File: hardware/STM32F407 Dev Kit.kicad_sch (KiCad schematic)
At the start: 0 parts

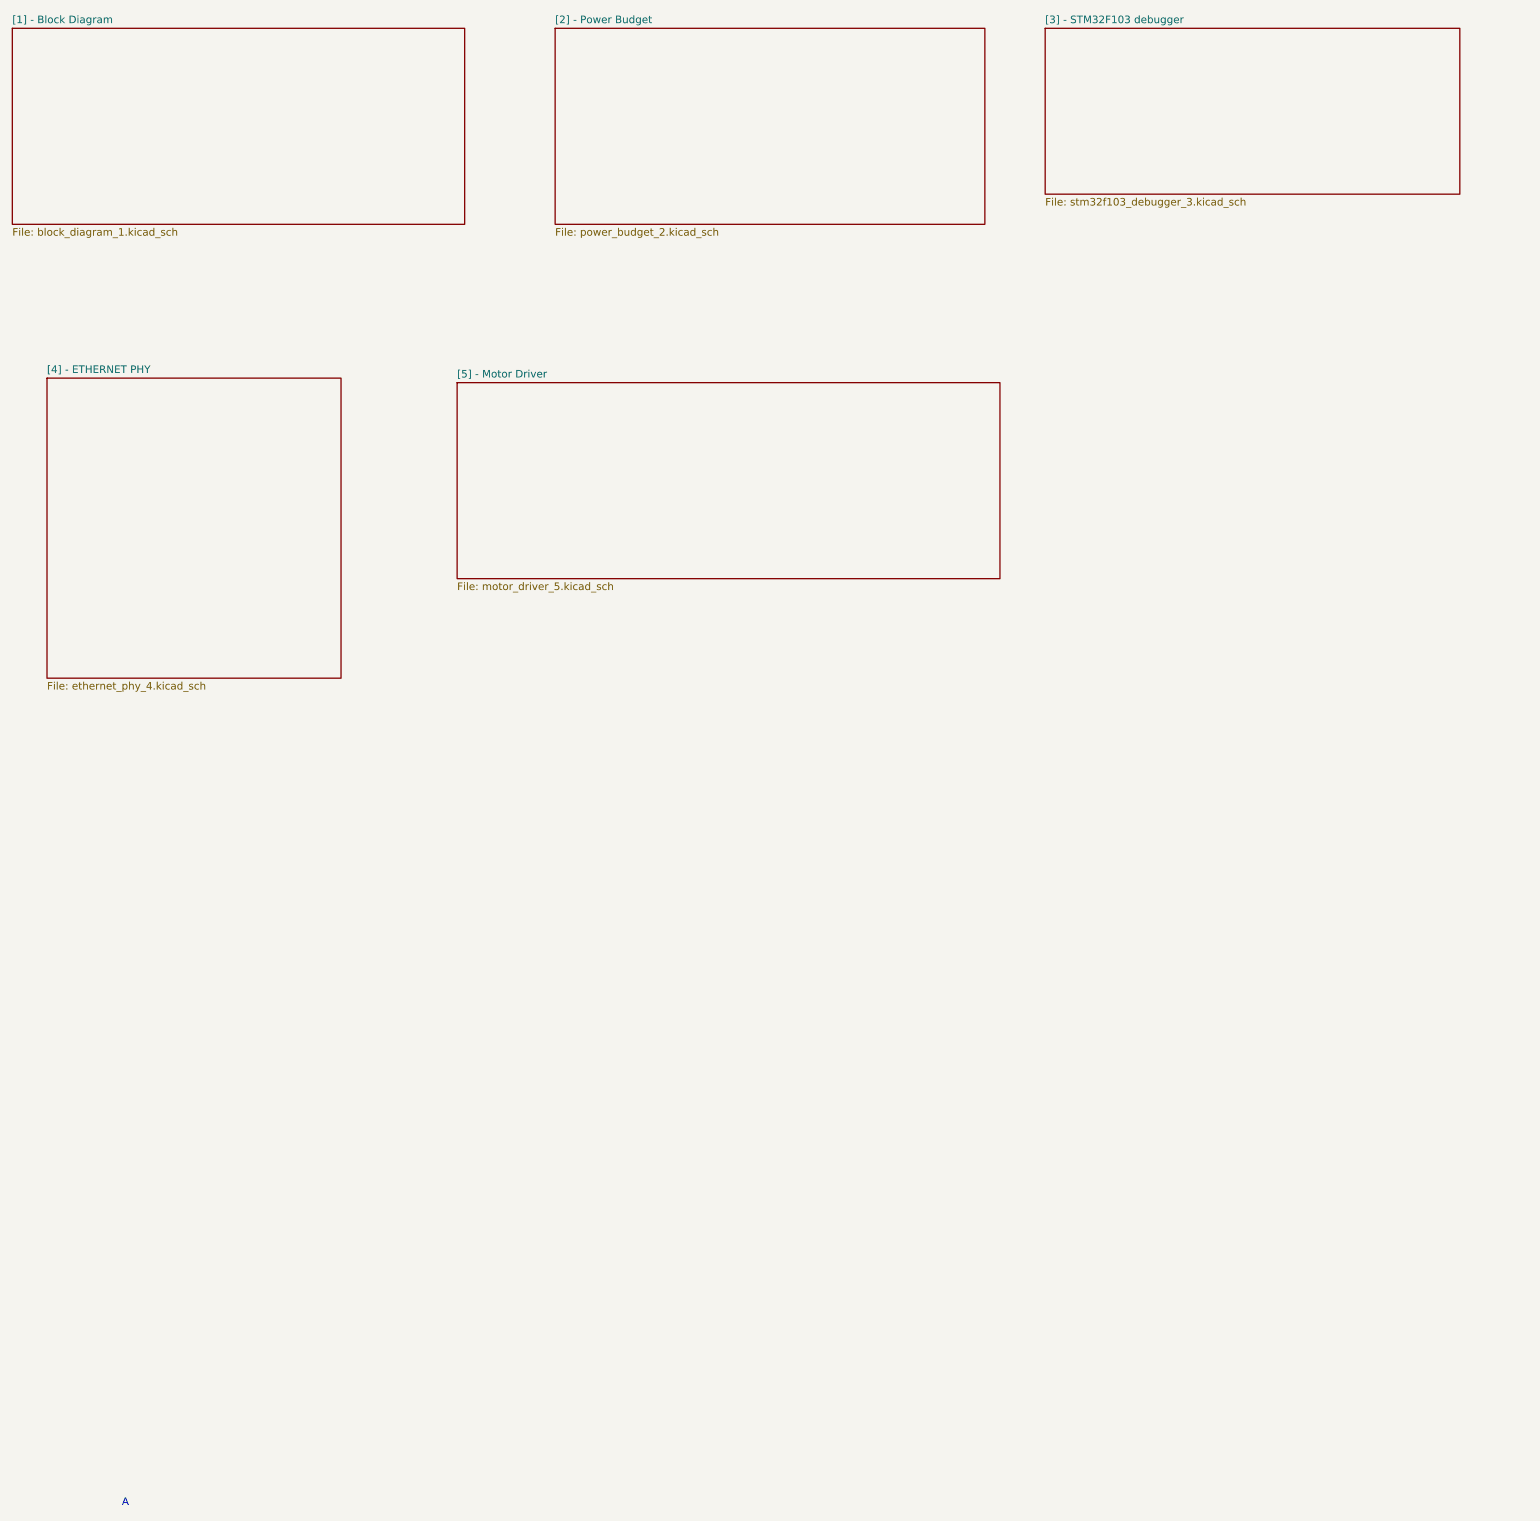
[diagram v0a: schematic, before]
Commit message: Design schematic for MIC & Headphones
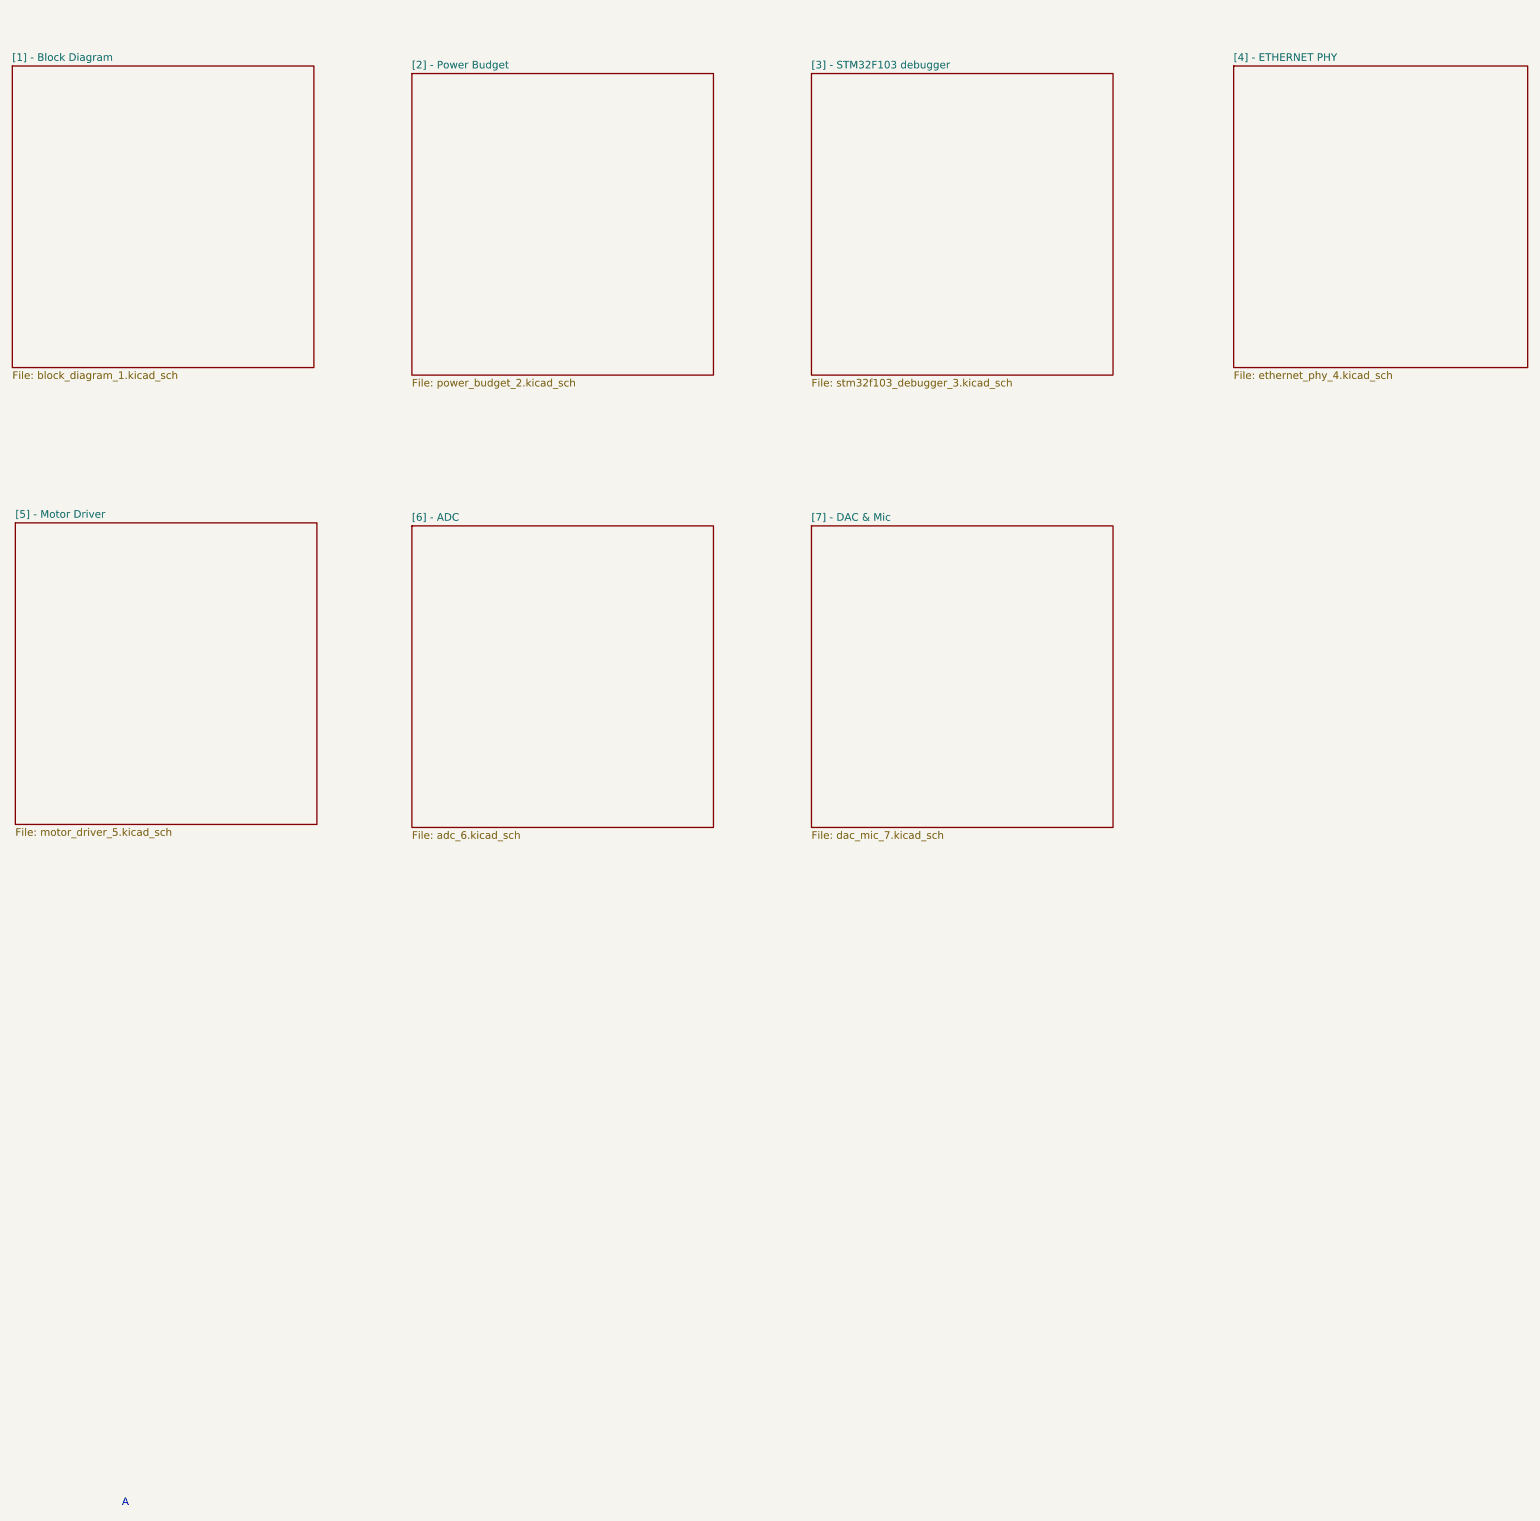
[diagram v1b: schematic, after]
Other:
- added sheet [6] - ADC (adc_6.kicad_sch)
- added sheet [7] - DAC & Mic (dac_mic_7.kicad_sch)
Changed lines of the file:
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@@
 	)
 	(sheet
-		(at 20.32 17.78)
-		(size 76.2 33.02)
+		(at 20.32 24.13)
+		(size 50.8 50.8)
 		(exclude_from_sim no)
 		(in_bom yes)
@@
 		)
 		(property "Sheetname" "[1] - Block Diagram"
-			(at 20.32 17.0684 0)
+			(at 20.32 23.4184 0)
 			(show_name no)
 			(do_not_autoplace no)
@@
 		)
 		(property "Sheetfile" "block_diagram_1.kicad_sch"
-			(at 20.32 51.3846 0)
+			(at 20.32 75.5146 0)
 			(show_name no)
 			(do_not_autoplace no)
@@
 	)
 	(sheet
-		(at 26.162 76.708)
-		(size 49.53 50.546)
+		(at 226.06 24.13)
+		(size 49.53 50.8)
 		(exclude_from_sim no)
 		(in_bom yes)
@@
 		)
 		(property "Sheetname" "[4] - ETHERNET PHY"
-			(at 26.162 75.9964 0)
+			(at 226.06 23.4184 0)
 			(show_name no)
 			(do_not_autoplace no)
@@
 		)
 		(property "Sheetfile" "ethernet_phy_4.kicad_sch"
-			(at 26.162 127.8386 0)
+			(at 226.06 75.5146 0)
 			(show_name no)
 			(do_not_autoplace no)
@@
 	)
 	(sheet
-		(at 111.76 17.78)
-		(size 72.39 33.02)
+		(at 154.94 101.6)
+		(size 50.8 50.8)
+		(exclude_from_sim no)
+		(in_bom yes)
+		(on_board yes)
+		(dnp no)
+		(fields_autoplaced yes)
+		(stroke
+			(width 0.1524)
+			(type solid)
+		)
+		(fill
+			(color 0 0 0 0)
+		)
+		(property "Sheetname" "[7] - DAC & Mic"
+			(at 154.94 100.8884 0)
+			(show_name no)
+			(do_not_autoplace no)
+			(effects
+				(font
+					(size 1.27 1.27)
+				)
+				(justify left bottom)
+			)
+		)
+		(property "Sheetfile" "dac_mic_7.kicad_sch"
+			(at 154.94 152.9846 0)
+			(show_name no)
+			(do_not_autoplace no)
+			(effects
+				(font
+					(size 1.27 1.27)
+				)
+				(justify left top)
+			)
+		)
+		(instances
+			(project "STM32F407 Dev Kit"
+				(path "/f3d27387-fbda-4c9d-aea0-93d92d34cd17"
+					(page "8")
+				)
+			)
+		)
+	)
+	(sheet
+		(at 87.63 25.4)
+		(size 50.8 50.8)
 		(exclude_from_sim no)
 		(in_bom yes)
@@
 		)
 		(property "Sheetname" "[2] - Power Budget"
-			(at 111.76 17.0684 0)
+			(at 87.63 24.6884 0)
 			(show_name no)
 			(do_not_autoplace no)
@@
 		)
 		(property "Sheetfile" "power_budget_2.kicad_sch"
-			(at 111.76 51.3846 0)
+			(at 87.63 76.7846 0)
 			(show_name no)
 			(do_not_autoplace no)
@@
 	)
 	(sheet
-		(at 194.31 17.78)
-		(size 69.85 27.94)
+		(at 154.94 25.4)
+		(size 50.8 50.8)
 		(exclude_from_sim no)
 		(in_bom yes)
@@
 		)
 		(property "Sheetname" "[3] - STM32F103 debugger"
-			(at 194.31 17.0684 0)
+			(at 154.94 24.6884 0)
 			(show_name no)
 			(do_not_autoplace no)
@@
 		)
 		(property "Sheetfile" "stm32f103_debugger_3.kicad_sch"
-			(at 194.31 46.3046 0)
+			(at 154.94 76.7846 0)
 			(show_name no)
 			(do_not_autoplace no)
@@
 	)
 	(sheet
-		(at 95.25 77.47)
-		(size 91.44 33.02)
+		(at 20.828 101.092)
+		(size 50.8 50.8)
 		(exclude_from_sim no)
 		(in_bom yes)
@@
 		)
 		(property "Sheetname" "[5] - Motor Driver"
-			(at 95.25 76.7584 0)
+			(at 20.828 100.3804 0)
 			(show_name no)
 			(do_not_autoplace no)
@@
 		)
 		(property "Sheetfile" "motor_driver_5.kicad_sch"
-			(at 95.25 111.0746 0)
+			(at 20.828 152.4766 0)
 			(show_name no)
 			(do_not_autoplace no)
@@
 				)
 			)
+		)
+	)
+	(sheet
+		(at 87.63 101.6)
+		(size 50.8 50.8)
+		(exclude_from_sim no)
+		(in_bom yes)
+		(on_board yes)
+		(dnp no)
+		(fields_autoplaced yes)
+		(stroke
+			(width 0.1524)
+			(type solid)
+		)
+		(fill
+			(color 0 0 0 0)
+		)
+		(property "Sheetname" "[6] - ADC"
+			(at 87.63 100.8884 0)
+			(show_name no)
+			(do_not_autoplace no)
+			(effects
+				(font
+					(size 1.27 1.27)
+				)
+				(justify left bottom)
+			)
+		)
+		(property "Sheetfile" "adc_6.kicad_sch"
+			(at 87.63 152.9846 0)
+			(show_name no)
+			(do_not_autoplace no)
+			(effects
+				(font
+					(size 1.27 1.27)
+				)
+				(justify left top)
+			)
+		)
+		(instances
+			(project "STM32F407 Dev Kit"
+				(path "/f3d27387-fbda-4c9d-aea0-93d92d34cd17"
+					(page "7")
+				)
+			)
